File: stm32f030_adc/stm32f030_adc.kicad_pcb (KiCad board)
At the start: 2 copper layers, 46 parts, among them Q1 BC337, U1 STM32F103C6Tx, U2 AMS1117-3.3, X1 USB_B_Micro, Y2 8 MHz

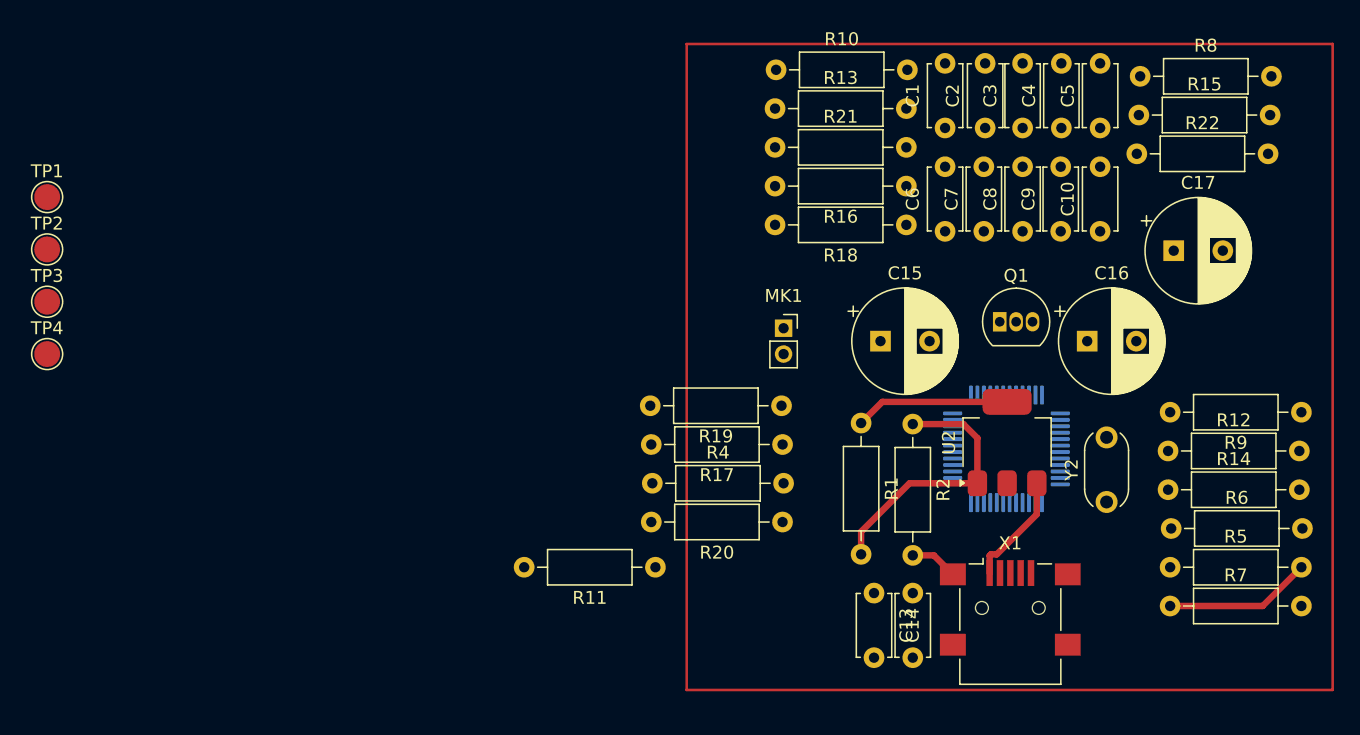
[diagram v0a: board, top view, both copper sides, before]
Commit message: [schematics] Impl |  Finished placement on "Vert" version
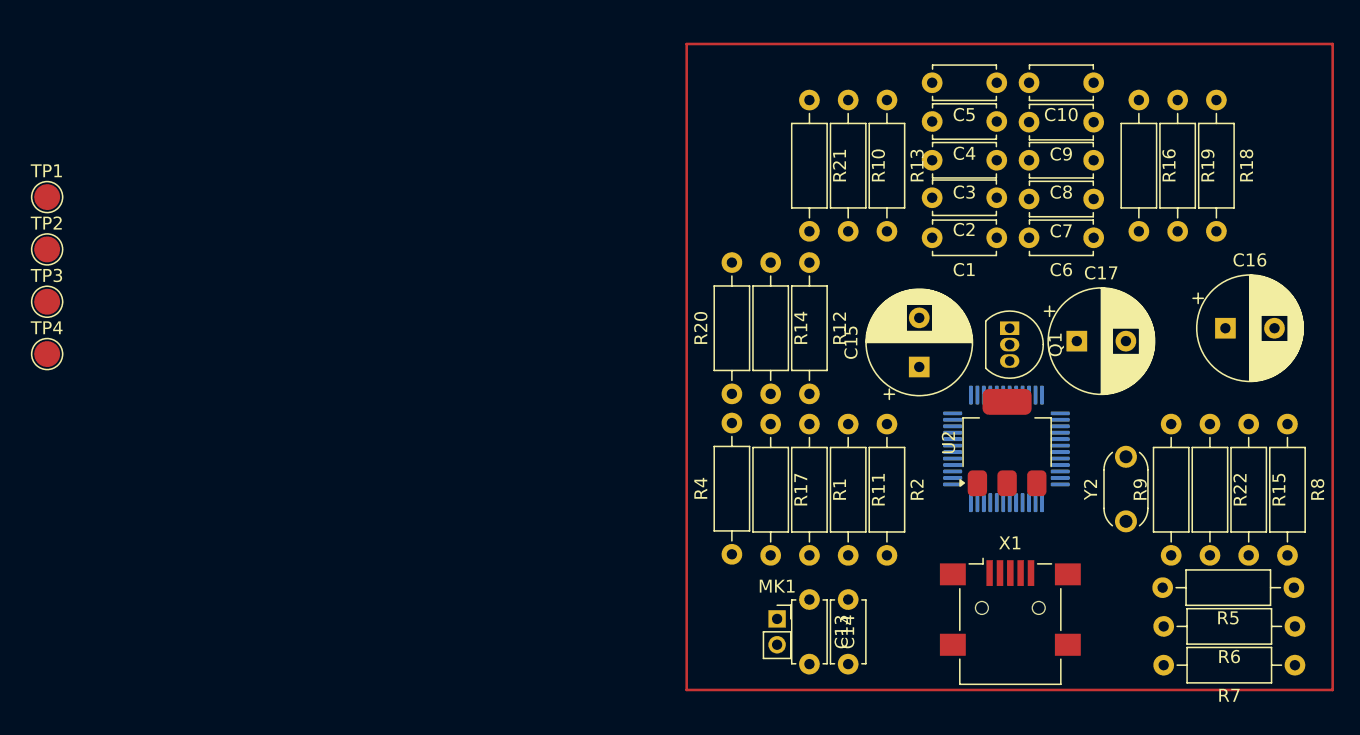
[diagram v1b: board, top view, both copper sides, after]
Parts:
- moved R19 38.7 mm to (218.5, 69.8), turned to -90 degrees
- moved R14 35.4 mm to (187.0, 82.4), turned to -90 degrees
- moved R12 31.4 mm to (190.0, 82.4), turned to -90 degrees
- moved R8 29.2 mm to (227.0, 94.9), turned to -90 degrees
- moved R18 25.9 mm to (221.5, 69.8), turned to -90 degrees
- moved R15 25.4 mm to (224.0, 94.9), turned to -90 degrees
- moved MK1 22.5 mm to (187.5, 110.0)
- moved R22 21.7 mm to (221.0, 94.9), turned to -90 degrees
- moved R16 19.2 mm to (215.5, 69.8), turned to -90 degrees
- moved R11 18.6 mm to (193.0, 94.9), turned to -90 degrees
- moved R9 15.0 mm to (218.0, 105.1), turned to 90 degrees
- moved R6 12.2 mm to (227.6, 110.6), turned to 180 degrees
- moved C10 11.5 mm to (212.0, 68.5), turned to 180 degrees
- moved C6 11.5 mm to (212.0, 80.5), turned to 180 degrees
- moved C16 10.7 mm to (222.2, 87.5)
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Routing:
- net Net-(U2-ADJ): track 21.3 -> 0.00 mm
- net +3V3: track 12.0 -> 0.00 mm
- net /Power and MCU/USB_D+: track 11.4 -> 0.00 mm
- net 5V_USB: track 8.73 -> 0.00 mm
- net GNDREF: track 3.71 -> 0.00 mm
